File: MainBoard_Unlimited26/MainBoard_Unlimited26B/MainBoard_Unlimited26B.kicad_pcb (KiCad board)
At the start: 2 copper layers, 95 x 60 mm, 48 parts, among them J1 power, J2 Conn_01x03_Pin, U1 TA6586, U10 TA6586, U2 TA6586, U3 TA6586, U4 TA6586, U5 TA6586, U7 ZC323000, U8 MP1584_3A_Mini

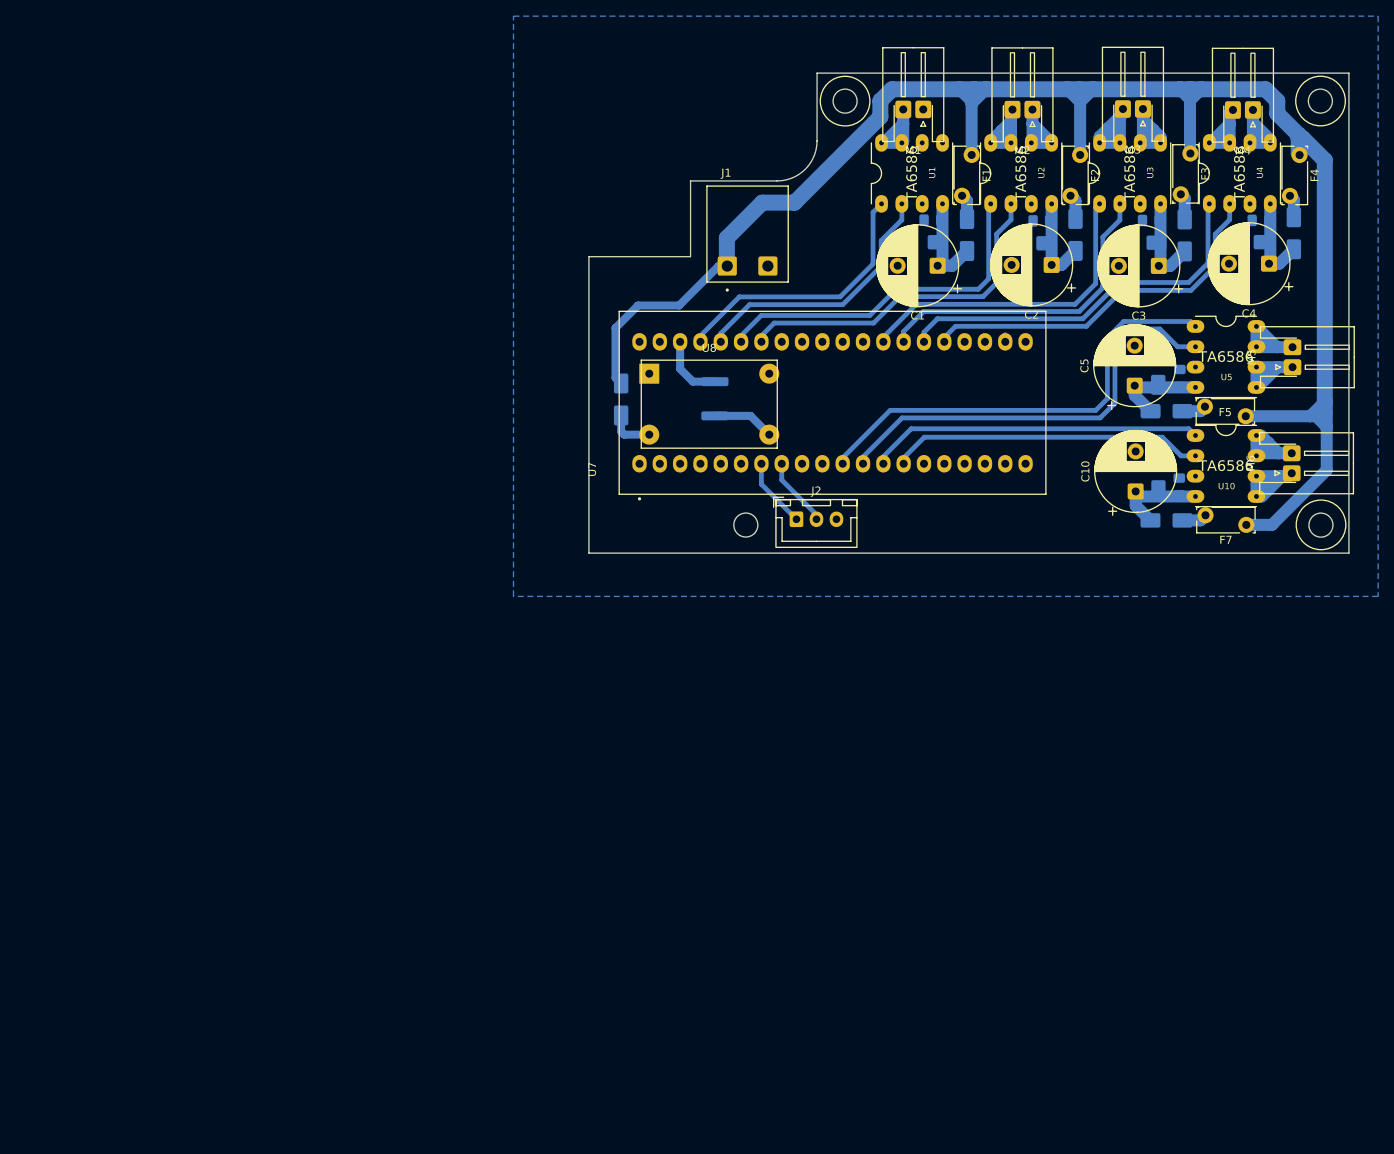
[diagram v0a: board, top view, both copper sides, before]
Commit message: REV ALL
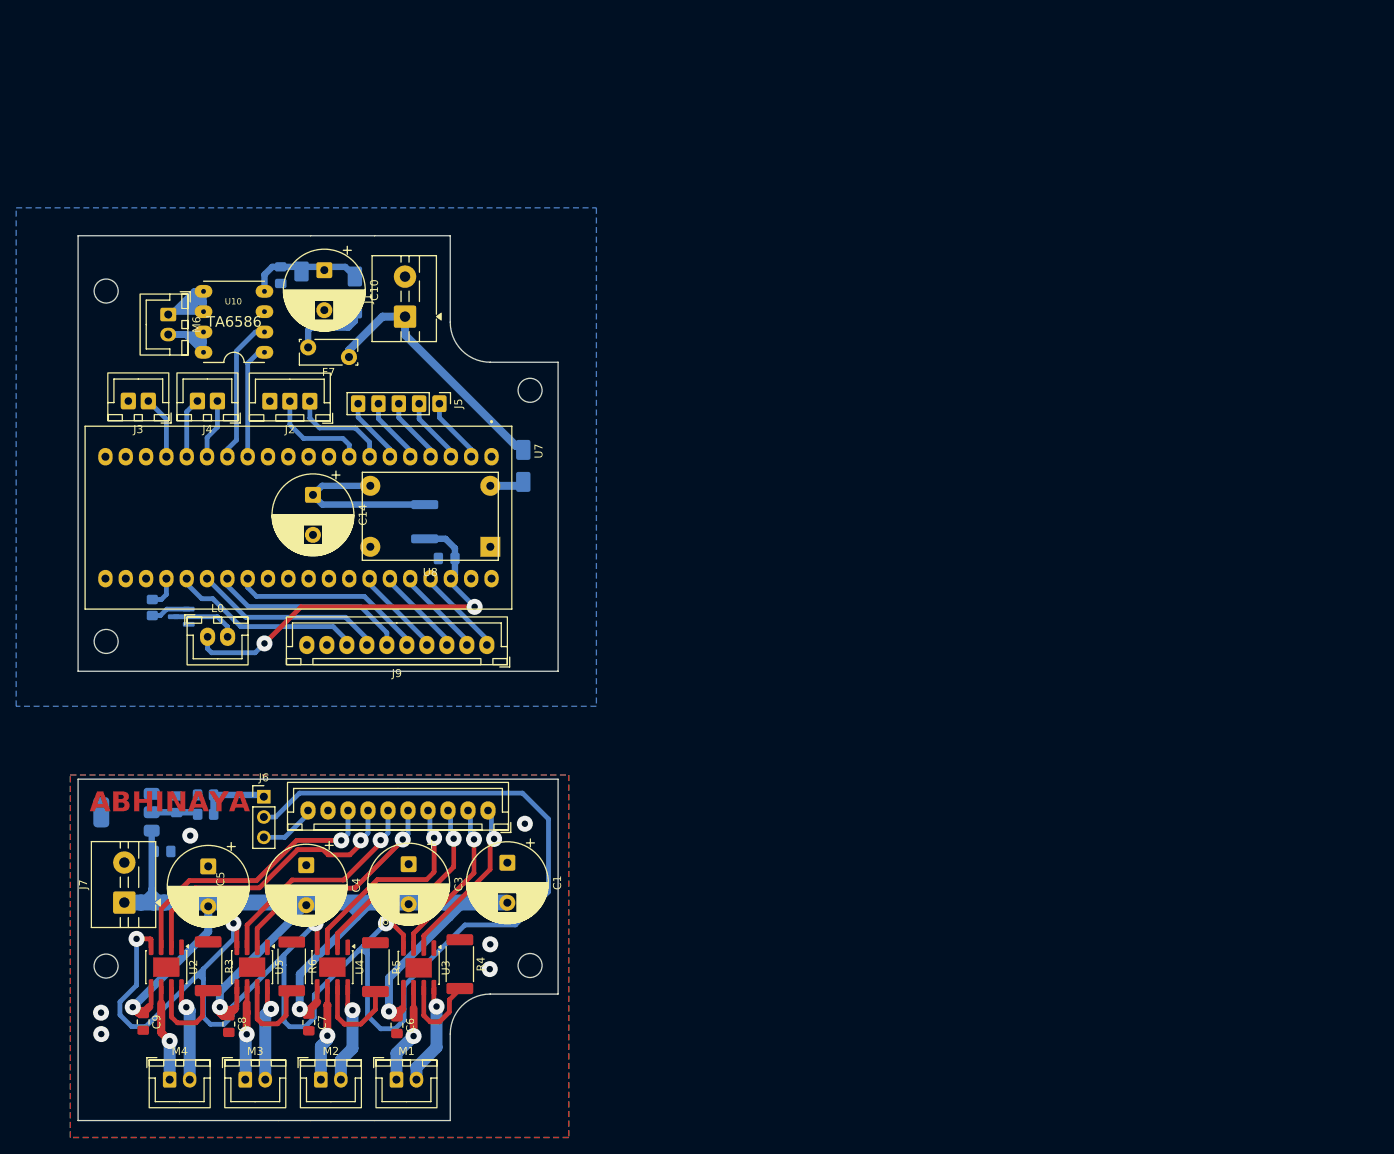
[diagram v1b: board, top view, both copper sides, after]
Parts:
- removed D1, D10, D2, D3, D4, D5, D6, D7, D8, D9: D_Schottky, Diode_SMD:D_SMA
- removed F1, F2, F3, F4, F5: Polyfuse, Fuse:Fuse_Bourns_MF-RG300
- removed M5: ~, Connector_JST:JST_XH_S2B-XH-A-1_1x02_P2.50mm_Horizontal
- added C13: 0.1uF, Capacitor_SMD:C_0805_2012Metric_Pad1.18x1.45mm_HandSolder, B.Cu at (145.0, 81.9)
- added C14: 1000uF, Capacitor_THT:CP_Radial_D10.0mm_P5.00mm, F.Cu at (128.2, 74.0)
- added J3: ~, Connector_JST:JST_XH_B2B-XH-A_1x02_P2.50mm_Vertical, F.Cu at (107.7, 62.2)
- added J4: ~, Connector_JST:JST_XH_B2B-XH-A_1x02_P2.50mm_Vertical, F.Cu at (116.3, 62.2)
- added J5: Conn_01x05_Pin, Connector_PinHeader_2.54mm:PinHeader_1x05_P2.54mm_Vertical, F.Cu at (144.1, 62.6)
- added J6: vreff mode, Connector_PinHeader_2.54mm:PinHeader_1x03_P2.54mm_Vertical, F.Cu at (122.1, 111.7)
- added J7: power, TerminalBlock:TerminalBlock_MaiXu_MX126-5.0-02P_1x02_P5.00mm, F.Cu at (104.7, 124.9)
- added J8: mconn, Connector_JST:JST_XH_B10B-XH-A_1x10_P2.50mm_Vertical, F.Cu at (150.1, 113.4)
- added J9: mconn, Connector_JST:JST_XH_B10B-XH-A_1x10_P2.50mm_Vertical, F.Cu at (150.0, 92.7)
- added L0: ~, Connector_JST:JST_XH_B2B-XH-A_1x02_P2.50mm_Vertical, F.Cu at (115.1, 91.7)
- added Q1: BC846, Package_TO_SOT_SMD:SOT-23, B.Cu at (111.8, 89.2)
- added R1: 10k, Resistor_SMD:R_0805_2012Metric_Pad1.20x1.40mm_HandSolder, B.Cu at (114.8, 113.9)
- added R2: 6k8, Resistor_SMD:R_0805_2012Metric_Pad1.20x1.40mm_HandSolder, B.Cu at (114.8, 111.5)
- added R3: 0.1, Resistor_SMD:R_2512_6332Metric_Pad1.40x3.35mm_HandSolder, F.Cu at (115.1, 132.9)
- added R4: 0.1, Resistor_SMD:R_2512_6332Metric_Pad1.40x3.35mm_HandSolder, F.Cu at (146.6, 132.6)
- added R5: 0.1, Resistor_SMD:R_2512_6332Metric_Pad1.40x3.35mm_HandSolder, F.Cu at (136.1, 133.0)
- added R6: 0.1, Resistor_SMD:R_2512_6332Metric_Pad1.40x3.35mm_HandSolder, F.Cu at (125.6, 132.9)
- added R7: 4k7, Resistor_SMD:R_0805_2012Metric_Pad1.20x1.40mm_HandSolder, B.Cu at (108.2, 88.1)
- C11: value 0.1uF -> 10uF
- C2: value 1000uF -> 10uF; footprint Capacitor_THT:CP_Radial_D10.0mm_P5.00mm -> Capacitor_SMD:C_0805_2012Metric_Pad1.18x1.45mm_HandSolder; moved to B.Cu
- C6, C7, C8, C9: value 0.1uF -> 100nF; moved to F.Cu
- J1: footprint terminal block right angel:TE_282815-2 -> TerminalBlock:TerminalBlock_MaiXu_MX126-5.0-02P_1x02_P5.00mm
- M1, M2, M3, M4, M6: footprint Connector_JST:JST_XH_S2B-XH-A-1_1x02_P2.50mm_Horizontal -> Connector_JST:JST_XH_B2B-XH-A_1x02_P2.50mm_Vertical
- U1: value TA6586 -> AMS1117-5.0; footprint TA6586:TA6586-FOOTPRINT -> Package_TO_SOT_SMD:SOT-223-3_TabPin2; moved to B.Cu
- U2, U3, U4, U5: value TA6586 -> A4950E; footprint TA6586:TA6586-FOOTPRINT -> Package_SO:SOIC-8-1EP_3.9x4.9mm_P1.27mm_EP2.41x3.3mm
- moved M4 181.7 mm to (110.3, 147.1), turned to 0 degrees
- moved C9 171.9 mm to (107.0, 139.9), turned to -90 degrees
- moved M3 165.3 mm to (119.8, 147.1), turned to 0 degrees
- moved U4 158.5 mm to (130.7, 133.0), turned to -90 degrees
- moved U2 153.8 mm to (109.9, 133.0), turned to -90 degrees
- moved C8 152.9 mm to (117.7, 140.1), turned to -90 degrees
- moved M2 150.4 mm to (129.2, 147.1), turned to 0 degrees
- moved U5 150.0 mm to (120.6, 133.0), turned to -90 degrees
- moved U10 143.6 mm to (109.5, 49.8), turned to 180 degrees
- moved C4 141.9 mm to (127.4, 120.3), turned to -90 degrees
- moved M6 141.8 mm to (110.2, 51.4), turned to -90 degrees
- moved U3 141.7 mm to (141.5, 133.1), turned to -90 degrees
- moved M1 138.0 mm to (138.7, 147.1), turned to 0 degrees
- moved C11 136.3 mm to (111.2, 112.7)
- moved C7 135.7 mm to (127.7, 139.9), turned to -90 degrees
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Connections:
- C1 pad 1: Net-(D1-K) -> GND
- C1 pad 2: GND -> +12V
- C11 pad 1: Net-(D10-K) -> Net-(U1-VO)
- C2 pad 1: Net-(D2-K) -> +12V
- C3 pad 1: Net-(D3-K) -> GND
- C3 pad 2: GND -> +12V
- C4 pad 1: Net-(D4-K) -> GND
- C4 pad 2: GND -> +12V
- C5 pad 1: Net-(D10-K) -> GND
- C5 pad 2: GND -> +12V
- C6 pad 1: Net-(D1-K) -> +12V
- C7 pad 1: Net-(D2-K) -> +12V
- C8 pad 1: Net-(D3-K) -> +12V
- C9 pad 1: Net-(D4-K) -> +12V
- D13 pad 2: +12V -> +12Vs
- F7 pad 1: +12V -> +12Vs
- J1 pad 1: +12V -> +12Vs
- M1 pad 1: F1 -> 1O1
- M1 pad 2: B1 -> 1O2
- M2 pad 1: F2 -> 2O1
- M2 pad 2: B2 -> 2O2
- M3 pad 1: F3 -> 3O1
- M3 pad 2: B3 -> 3O2
- M4 pad 1: F4 -> 4O1
- M4 pad 2: B4 -> 4O2
- U7 pad 10: unconnected-(U7-A5-Pad10) -> DA5
- U7 pad 15: unconnected-(U7-B10-Pad15) -> PB10
- U7 pad 16: unconnected-(U7-B11-Pad16) -> PB11
- U7 pad 17: unconnected-(U7-R-Pad17) -> R
- U7 pad 2: unconnected-(U7-C13-Pad2) -> PC13
- U7 pad 21: unconnected-(U7-B12-Pad21) -> DB12
- U7 pad 22: unconnected-(U7-B13-Pad22) -> DB13
- U7 pad 23: unconnected-(U7-B14-Pad23) -> DB14
- U7 pad 24: unconnected-(U7-B15-Pad24) -> DB15
- U7 pad 3: unconnected-(U7-C14-Pad3) -> PC14
- U7 pad 33: unconnected-(U7-B5-Pad33) -> DB5
- U7 pad 4: unconnected-(U7-C15-Pad4) -> PC15
- U7 pad 9: unconnected-(U7-A4-Pad9) -> DA4
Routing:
- net REFF: track 0.00 -> 194.0 mm, vias 0 -> 4
- net PA6: track 56.6 -> 0.00 mm
- net PA7: track 54.5 -> 0.00 mm
- net +12V: track 221.8 -> 171.4 mm, vias 0 -> 4
- net +5V: track 8.39 -> 50.7 mm, vias 0 -> 2
- net +12Vs: track 0.00 -> 32.2 mm
- net PB0: track 41.7 -> 14.3 mm
- net PB1: track 39.3 -> 18.2 mm
- net F3: track 14.4 -> 0.00 mm
- net Net-(U8-VOUT+): track 7.77 -> 22.1 mm
- net B3: track 13.7 -> 0.00 mm
- net 1O1: track 0.00 -> 13.6 mm, vias 0 -> 1
- net PA11: track 40.1 -> 53.6 mm, vias 0 -> 1
- net PA10: track 39.8 -> 53.0 mm, vias 0 -> 1
- net PA9: track 47.8 -> 60.6 mm, vias 0 -> 1
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- added copper zone on F.Cu, net GND
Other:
- board size 95 x 60 mm -> 60 x 110.6 mm
- board text added: "ABHINAYA"
